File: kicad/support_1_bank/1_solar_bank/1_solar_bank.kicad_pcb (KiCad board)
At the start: 2 copper layers, 88.9 x 94 mm, 32 parts, among them J1 Conn_01x09, M1 VN10KM, M2 BS250, M3 VN10KM, M4 BS250

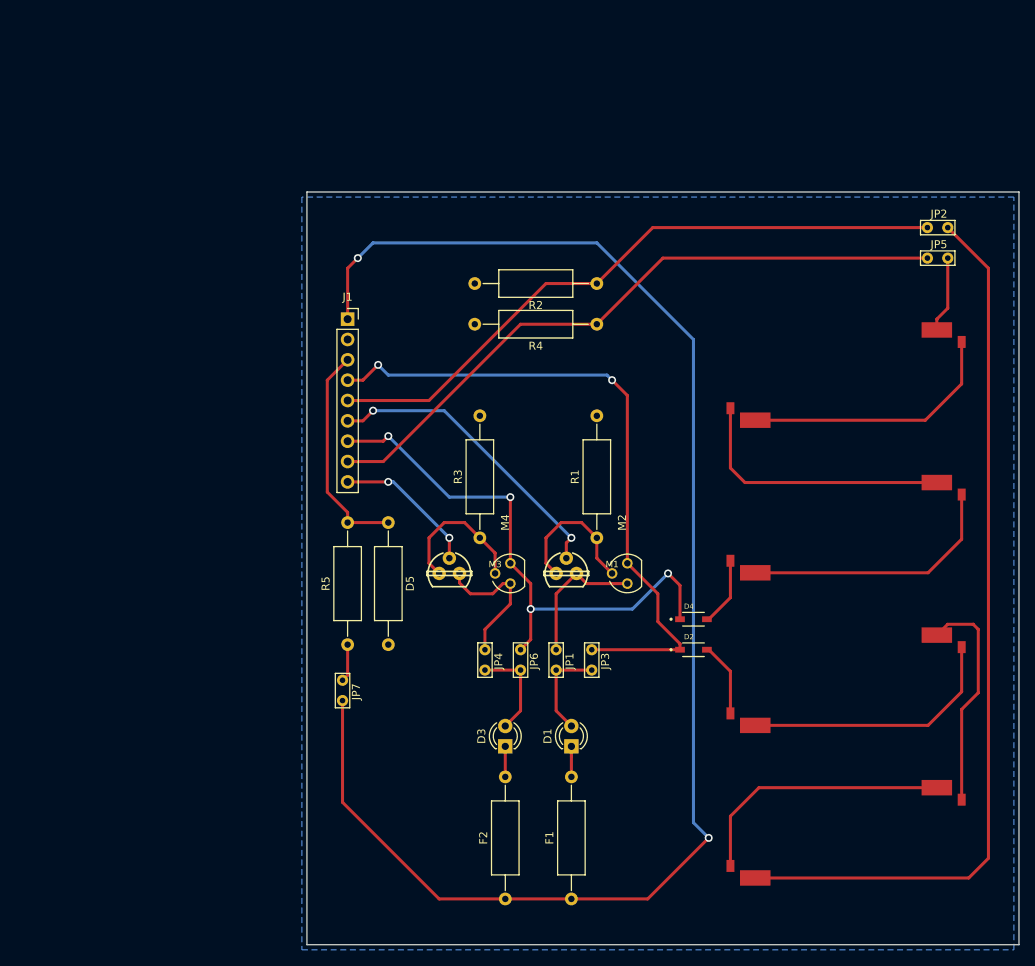
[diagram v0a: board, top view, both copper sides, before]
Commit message: revision schemas + pcb
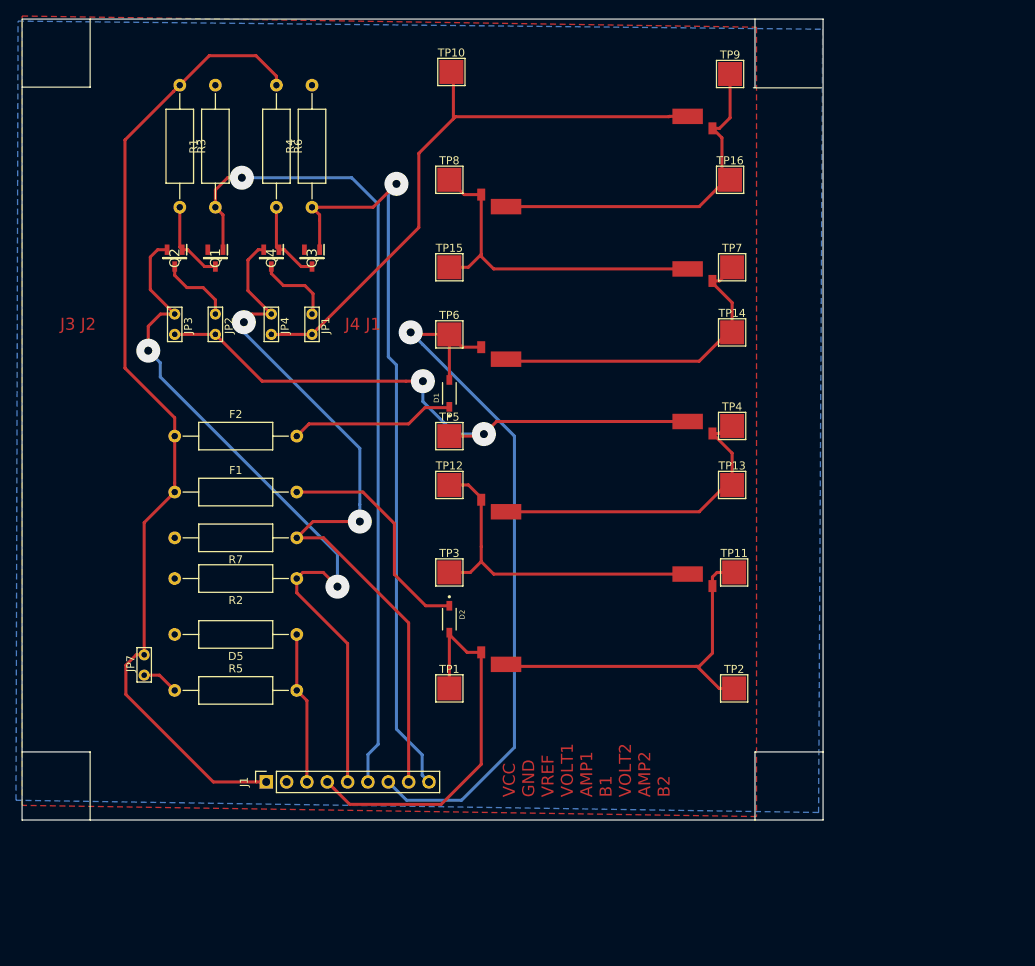
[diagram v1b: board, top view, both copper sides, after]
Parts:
- removed D3: LED, panneaux_solaires:LED_D3.0mm
- removed D4: D_Schottky, panneaux_solaires:SOD3715X135N
- removed JP5, JP6: Jumper_2_Bridged, panneaux_solaires:TestPoint_Bridge_Pitch2.54mm_Drill0.7mm
- removed M1, M3: VN10KM, panneaux_solaires:TO237
- removed M2, M4: BS250, panneaux_solaires:SOT54E
- added Q1: RUR040N02HZGTL, panneaux_solaires:RUR040N02HZGTL, F.Cu at (74.9, 48.9)
- added Q2: RUR040N02HZGTL, panneaux_solaires:RUR040N02HZGTL, F.Cu at (69.8, 48.9)
- added Q3: RUR040N02HZGTL, panneaux_solaires:RUR040N02HZGTL, F.Cu at (87.0, 48.9)
- added Q4: RUR040N02HZGTL, panneaux_solaires:RUR040N02HZGTL, F.Cu at (81.9, 48.9)
- added R6: 1M, panneaux_solaires:R_Axial_DIN0309_L9.0mm_D3.2mm_P15.24mm_Horizontal, F.Cu at (82.5, 27.3)
- added R7: 20R, panneaux_solaires:R_Axial_DIN0309_L9.0mm_D3.2mm_P15.24mm_Horizontal, F.Cu at (85.1, 83.8)
- added TP1: TestPoint, panneaux_solaires:TestPoint_Pad_3.0x3.0mm, F.Cu at (104.1, 102.6)
- added TP10: TestPoint, panneaux_solaires:TestPoint_Pad_3.0x3.0mm, F.Cu at (104.4, 25.7)
- added TP11: TestPoint, panneaux_solaires:TestPoint_Pad_3.0x3.0mm, F.Cu at (139.7, 88.1)
- added TP12: TestPoint, panneaux_solaires:TestPoint_Pad_3.0x3.0mm, F.Cu at (104.1, 77.2)
- added TP13: TestPoint, panneaux_solaires:TestPoint_Pad_3.0x3.0mm, F.Cu at (139.4, 77.2)
- added TP14: TestPoint, panneaux_solaires:TestPoint_Pad_3.0x3.0mm, F.Cu at (139.4, 58.2)
- added TP15: TestPoint, panneaux_solaires:TestPoint_Pad_3.0x3.0mm, F.Cu at (104.1, 50.0)
- added TP16: TestPoint, panneaux_solaires:TestPoint_Pad_3.0x3.0mm, F.Cu at (139.2, 39.1)
- added TP2: TestPoint, panneaux_solaires:TestPoint_Pad_3.0x3.0mm, F.Cu at (139.7, 102.6)
- added TP3: TestPoint, panneaux_solaires:TestPoint_Pad_3.0x3.0mm, F.Cu at (104.1, 88.1)
- added TP4: TestPoint, panneaux_solaires:TestPoint_Pad_3.0x3.0mm, F.Cu at (139.4, 69.8)
- added TP5: TestPoint, panneaux_solaires:TestPoint_Pad_3.0x3.0mm, F.Cu at (104.1, 71.1)
- added TP6: TestPoint, panneaux_solaires:TestPoint_Pad_3.0x3.0mm, F.Cu at (104.1, 58.4)
- added TP7: TestPoint, panneaux_solaires:TestPoint_Pad_3.0x3.0mm, F.Cu at (139.4, 50.0)
- added TP8: TestPoint, panneaux_solaires:TestPoint_Pad_3.0x3.0mm, F.Cu at (104.1, 39.1)
- added TP9: TestPoint, panneaux_solaires:TestPoint_Pad_3.0x3.0mm, F.Cu at (139.2, 25.9)
- D1: value LED -> D_Schottky; footprint panneaux_solaires:LED_D3.0mm -> panneaux_solaires:SOD3715X135N
- R1: value 1M -> 20R
- moved JP2 92.4 mm to (74.9, 58.4), turned to 90 degrees
- moved SC3 72.9 mm to (109.2, 75.6), turned to 180 degrees
- moved F2 71.0 mm to (69.8, 71.1), turned to 0 degrees
- moved F1 70.9 mm to (69.8, 78.1), turned to 0 degrees
- moved R3 67.8 mm to (70.5, 27.3), turned to 270 degrees
- moved JP3 66.8 mm to (69.8, 58.4)
- moved R1 63.0 mm to (74.9, 42.5)
- moved J1 58.7 mm to (81.3, 114.3), turned to 90 degrees
- moved R2 52.5 mm to (85.1, 88.9)
- moved JP1 51.8 mm to (87.0, 58.4)
- moved JP4 49.7 mm to (81.9, 58.4)
- moved SC4 47.2 mm to (135.9, 74.3), turned to 0 degrees
- moved D1 46.6 mm to (104.1, 65.8)
- moved SC6 41.0 mm to (135.9, 55.2)
- moved SC5 41.0 mm to (109.2, 56.5)
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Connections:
- D1 pad 2: Net-(D1-Pad2) -> VOLTMETER2
- D2 pad 1: VOLTMETER1 -> Net-(D2-Pad1)
- D2 pad 2: Net-(D2-Pad2) -> VOLTMETER1
- F1 pad 2: Net-(D1-Pad1) -> Net-(D2-Pad1)
- F2 pad 2: Net-(D3-Pad1) -> Net-(D1-Pad1)
- JP1 pad 1: Net-(D1-Pad2) -> Net-(JP1-Pad1)
- JP2 pad 2: AMPERMETER1 -> Net-(JP2-Pad2)
- JP3 pad 1: Net-(D1-Pad2) -> Net-(JP2-Pad1)
- JP3 pad 2: VOLTMETER1 -> AMPERMETER1
- JP4 pad 1: Net-(D3-Pad2) -> Net-(JP1-Pad1)
- JP4 pad 2: Net-(JP4-Pad2) -> AMPERMETER2
- R1 pad 1: Net-(M1-Pad3) -> BNK1_CONTROL
- R3 pad 1: Net-(M3-Pad3) -> +VSW
- R3 pad 2: GND -> Net-(Q1-Pad2)
- R4 pad 1: AMPERMETER2 -> BNK2_CONTROL
- SC1 pad 1: Net-(D2-Pad2) -> VOLTMETER1
- SC5 pad 1: Net-(D4-Pad2) -> VOLTMETER2
- SC8 pad 2: Net-(JP5-Pad1) -> Net-(JP1-Pad1)
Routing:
- net BNK2_CONTROL: track 18.1 -> 94.6 mm
- net Net-(JP1-Pad1): track 0.00 -> 74.6 mm
- net BNK1_CONTROL: track 37.8 -> 102.8 mm, vias 2 -> 1
- net +VSW: track 185.4 -> 122.4 mm, vias 2 -> 0
- net Net-(JP2-Pad1): track 111.0 -> 75.8 mm, vias 0 -> 2
- net VOLTMETER1: track 82.8 -> 48.5 mm, vias 2 -> 0
- net Net-(D2-Pad1): track 0.00 -> 28.6 mm
- net VOLTMETER2: track 69.7 -> 92.9 mm, vias 4 -> 1
- net Net-(JP4-Pad2): track 18.2 -> 0.00 mm
- net Net-(M3-Pad3): track 18.1 -> 0.00 mm
- net Net-(M1-Pad3): track 18.1 -> 0.00 mm
- net Net-(D1-Pad1): track 3.81 -> 20.5 mm
- net Net-(SC2-Pad2): track 28.1 -> 43.6 mm
- net Net-(D3-Pad2): track 12.2 -> 0.00 mm
- net Net-(D1-Pad2): track 12.2 -> 0.00 mm
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- added copper zone on F.Cu, net GND
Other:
- board size 88.9 x 94 mm -> 100 x 100 mm
- board text added: "J3 J2"
- board text added: "J4 J1"
- board text added: "VCC GND VREF VOLT1 AMP1 B1 VOLT2 AMP2 B2"
